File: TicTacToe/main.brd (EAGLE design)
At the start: 127 x 97.5 mm, 23 parts, among them U1 AT90USB1286-AU, Y1 16MHz

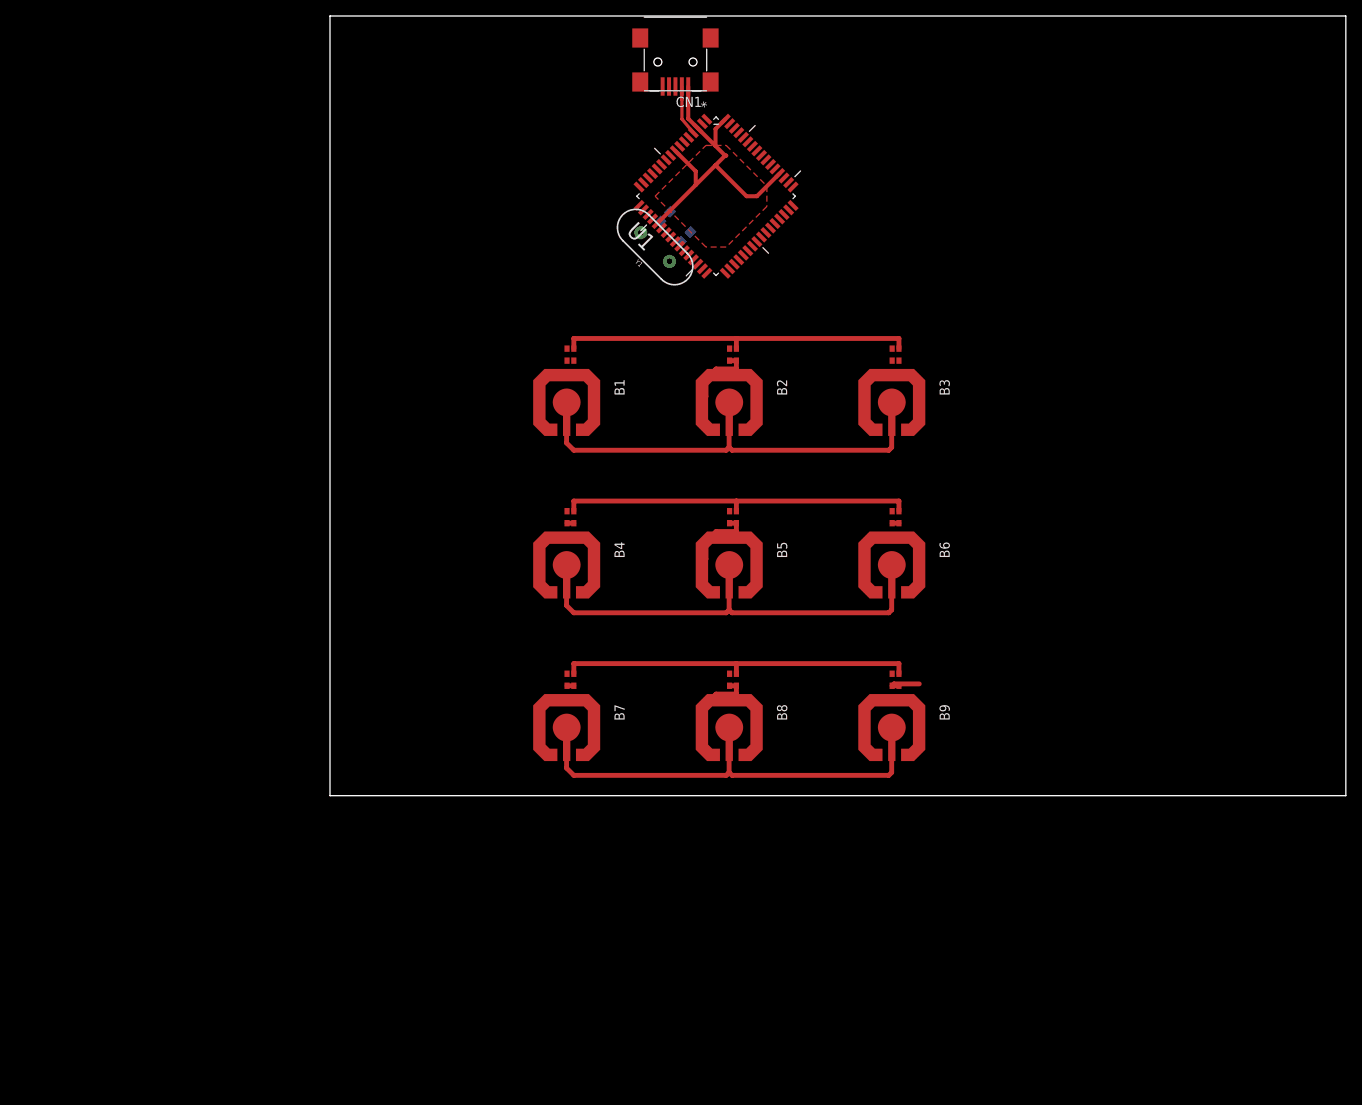
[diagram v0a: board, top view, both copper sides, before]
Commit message: ttt
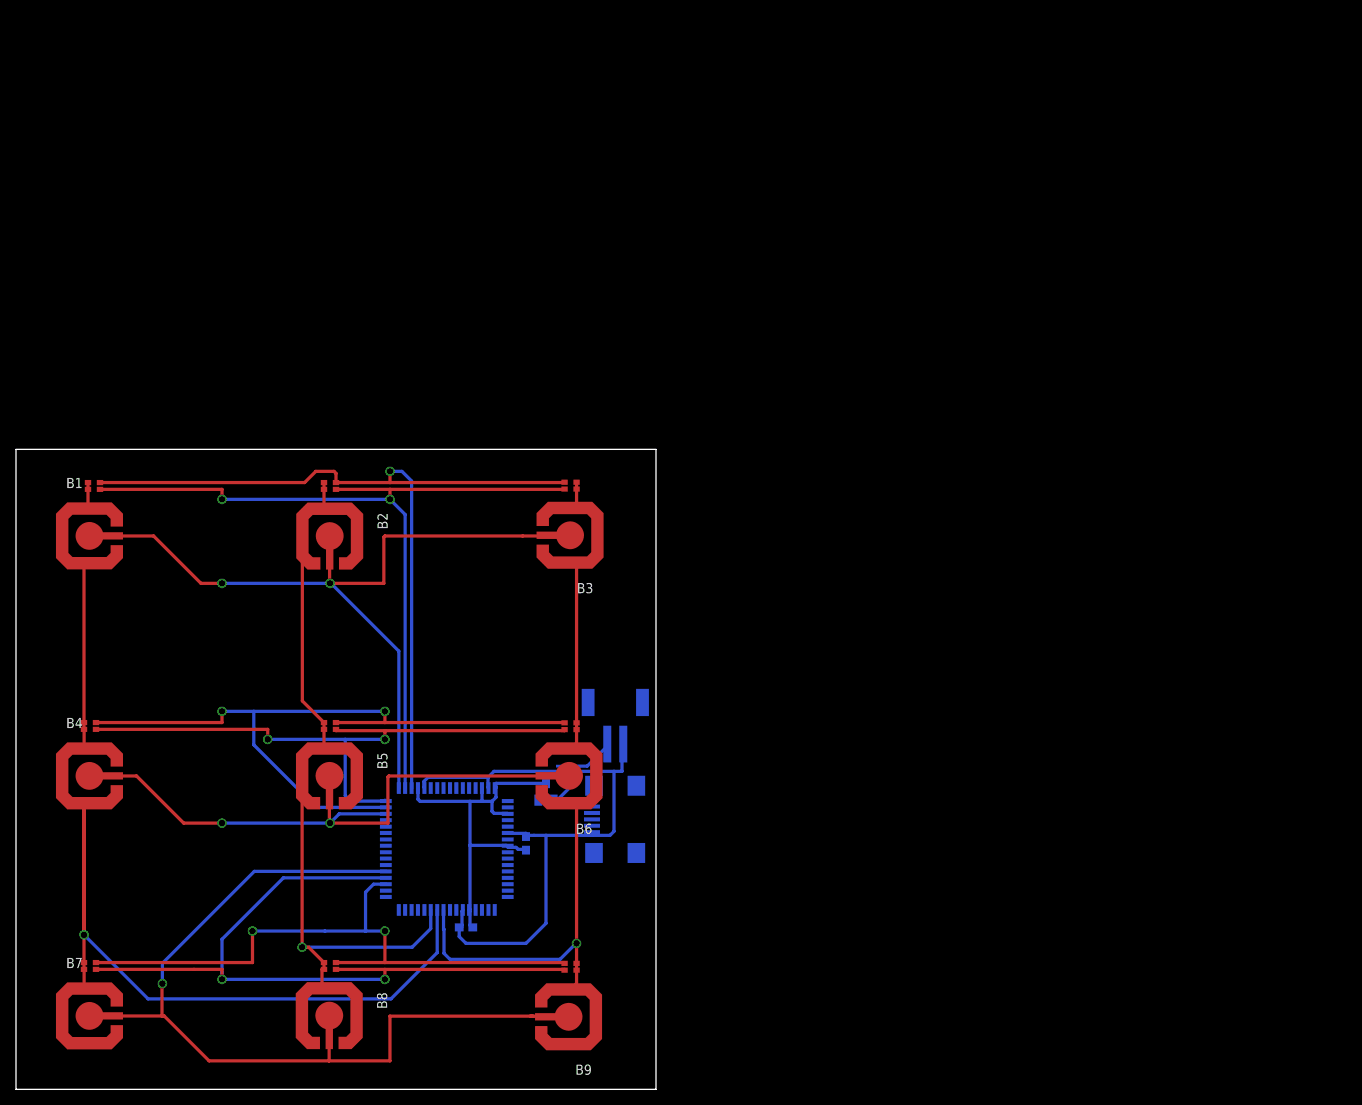
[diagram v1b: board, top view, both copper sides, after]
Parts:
- removed CN1: (no value), adafruit:USB-MINIB
- removed Y1: 16MHz, SparkFun-Clocks:HC49US
- added D1: BAT54, diode:SOT23
- added J1: (no value), SparkFun-Connectors:JST-2-SMD
- added U$1: MIC94090, 7_segment_lib:SC70-6L
- added X2: MINI-USB-SHIELD-UX60A-MB-5ST, con-hirose:UX60A-MB-5ST
- C1, C2: value 10p -> 100n
- moved L1 97.9 mm to (-29.2, -24.2), turned to 180 degrees
- moved L2 92.3 mm to (0.75, -24.2), turned to 180 degrees
- moved C1 90.6 mm to (17.0, -19.0), turned to 0 degrees
- moved U1 88.3 mm to (14.6, -9.21), flipped to the bottom, turned to 0 degrees
- moved L3 87.5 mm to (29.3, -23.5), turned to 0 degrees
- moved C2 80.3 mm to (24.5, -8.50), turned to 90 degrees
- moved B7 74.4 mm to (-34.2, -34.2), turned to 0 degrees
- moved B4 69.0 mm to (-34.2, -4.25), turned to 0 degrees
- moved B1 64.7 mm to (-34.2, 25.8), turned to 0 degrees
- moved B8 61.6 mm to (-4.28, -25.8)
- moved L7 60.1 mm to (-29.2, 5.75), turned to 180 degrees
- moved L4 59.3 mm to (-28.8, 35.8), turned to 180 degrees
- moved B5 56.5 mm to (-4.25, 4.12)
- moved B2 52.7 mm to (-4.22, 34.1)
- moved L8 50.5 mm to (0.75, 5.75), turned to 180 degrees
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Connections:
- removed net ID: CN1.ID
- removed net X1: C1.1, U1.24, Y1.1
- removed net X2: C2.1, U1.23, Y1.2
- new net N$3: J1.NC2
- new net N$4: J1.NC1
- new net PA6: U1.45
- new net PA7: U1.44
- new net PB0: U1.10
- new net PB1: U1.11
- new net PB2: U1.12
- new net PB3: U1.13
- new net PB4: U1.14
- new net PB5: U1.15
- new net PB6: U1.16
- new net PB7: U1.17
- new net PC3: U1.38
- new net PC4: U1.39
- new net PC5: U1.40
- new net PC6: U1.41
- new net PC7: U1.42
- new net PD3: U1.28
- new net PD4: U1.29
- new net PD5: U1.30
- new net PD6: U1.31
- new net PD7: U1.32
- new net PE0: U1.33
- new net PE1: U1.34
- new net PE2: U1.43
- new net PE3: U1.9
- new net PE4: U1.18
- new net PE5: U1.19
- new net PE6: U1.1
- new net PE7: U1.2
- new net PF0: U1.61
- new net PF1: U1.60
- new net PF2: U1.59
- new net PF3: U1.58
- new net PF4: U1.57
- new net PF5: U1.56
- new net PF6: U1.55
- new net PF7: U1.54
- new net UCAP: U1.7
- new net USB: D1.1, U$1.6, X2.1
- new net VBAT: J1.2, U$1.4
- new net XTAL1: U1.24
- new net XTAL2: U1.23
- new net ~RESET: U1.20
- net C1: now also U1.26; no longer U1.10
- net C2: now also U1.27; no longer U1.11
- net C3: now also U1.25; no longer U1.12
- net D_N: no longer CN1.D-
- net D_P: no longer CN1.D+
- net GND: now also J1.1, U$1.2, U$1.5, X2.5; no longer CN1.GND
- net L11: now also L3.A2, U1.36; no longer L3.A1, U1.35
- net L12: now also L3.A1, U1.35; no longer L3.A2, U1.36
- net L1B: now also U1.49
- net L21: now also L6.A2, U1.50; no longer L6.A1, U1.37
- net L22: now also L6.A1, U1.51; no longer L6.A2, U1.38
- net L2B: now also U1.46
- net L31: now also L9.A2, U1.48; no longer L9.A1, U1.39
- net L32: now also L9.A1, U1.47; no longer L9.A2, U1.40
- net L3B: now also U1.37
- net VCC: now also C1.1, C2.1, D1.3, U$1.1, U1.62; no longer CN1.VBUS
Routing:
- net C1: track 1.70 -> 177.9 mm, vias 0 -> 1
- net L22: track 0.00 -> 102.9 mm, vias 0 -> 1
- net L32: track 0.00 -> 91.4 mm, vias 0 -> 2
- net C3: track 5.19 -> 95.9 mm, vias 0 -> 1
- net L12: track 0.00 -> 80.5 mm, vias 0 -> 2
- net GND: track 0.00 -> 80.3 mm
- net C2: track 27.3 -> 94.8 mm, vias 0 -> 1
- net L21: track 44.4 -> 104.2 mm, vias 0 -> 2
- net L3B: track 47.2 -> 102.5 mm, vias 0 -> 1
- net L11: track 44.4 -> 95.9 mm, vias 0 -> 2
- net L1B: track 47.2 -> 93.0 mm, vias 0 -> 2
- net L31: track 44.5 -> 79.9 mm, vias 0 -> 2
- net L2B: track 47.2 -> 71.0 mm, vias 0 -> 2
- net USB: track 0.00 -> 9.21 mm
- net VCC: track 42.8 -> 50.7 mm
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- removed copper zone on layer 1, net VCC
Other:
- board size 127 x 97.5 mm -> 80 x 80 mm
